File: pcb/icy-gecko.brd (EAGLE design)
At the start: 50.8 x 25.4 mm, 64 parts, among them J1 USB-C, J2 8, J3 8, J4 8, J5 8, J6 4, J7 4, U1 EFM32GG12B8XX_QFN64, U2 ICE40LP384-SG32, U3 MIC23159, U6 SST26VF016B

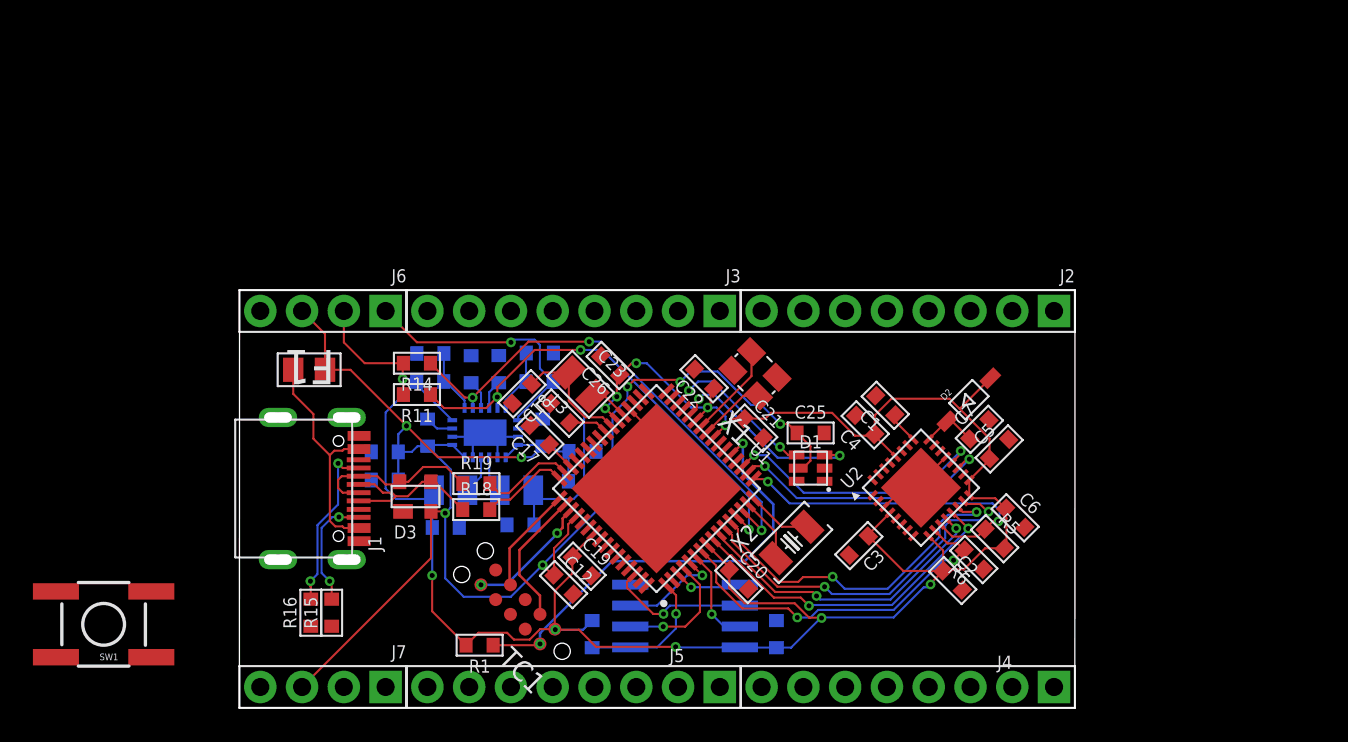
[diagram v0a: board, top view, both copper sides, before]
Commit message: pcd finito
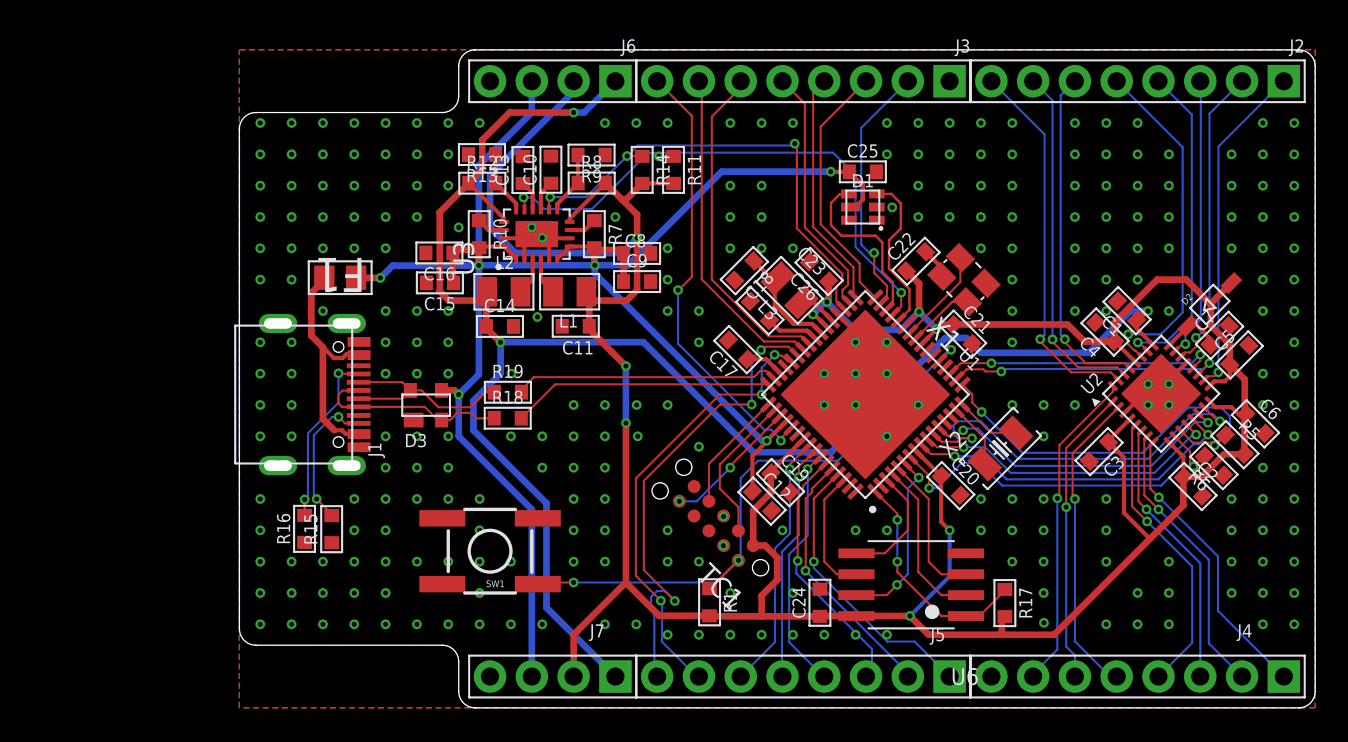
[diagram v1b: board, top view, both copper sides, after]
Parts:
- moved R17 25.2 mm to (46.5, 6.37), flipped to the top, turned to 270 degrees
- moved SW1 23.9 mm to (15.2, 9.53)
- moved R11 20.7 mm to (26.4, 32.7), turned to 270 degrees
- moved J2 19.8 mm to (61.0, 38.1)
- moved J3 19.8 mm to (40.6, 38.1)
- moved J6 19.8 mm to (20.3, 38.1)
- moved C8 19.5 mm to (24.2, 27.6), flipped to the top
- moved C9 19.5 mm to (24.2, 25.9), flipped to the top
- moved R14 18.0 mm to (24.5, 32.7), turned to 270 degrees
- moved C25 16.2 mm to (37.9, 32.6)
- moved D1 16.2 mm to (37.9, 30.4)
- moved C1 15.8 mm to (54.0, 24.1)
- moved R7 15.8 mm to (21.6, 28.8), flipped to the top
- moved D2 15.8 mm to (59.0, 24.5)
- moved C2 15.7 mm to (58.0, 13.5)
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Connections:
- net 1V2_PG: now also U1.29; no longer U1.13
- net 3V3_PG: now also U1.35; no longer U1.14
- net IOL_2A: now also J4.5
- net IOL_2B: now also J4.6
- net IOL_4A: now also J4.4
- net IOL_4B_GBIN7: now also J4.3
- net IOL_5A_GBIN6: now also J4.1
- net IOL_5B: now also J4.2
- net IOR_34: now also J2.1
- net IOR_38: now also J2.2
- net IOR_39: now also J2.3
- net IOT_45: now also J2.4
- net IOT_47: now also J2.5
- net IOT_49_GBIN0: now also J2.6
- net IOT_50_GBIN1: now also J2.7
- net IOT_52: now also J4.7
- net IOT_53: now also J2.8
- net PD3: now also J3.2
- net PD4: now also J3.3
- net PD5: now also J3.4
- net PD6: now also J3.5
- net PE10: now also J5.4
- net PE11: now also J5.3
- net PE12: now also J5.2
- net PE13: now also J5.1
- net PE4: now also J3.6
- net PE5: now also J3.7
- net PE6: now also J5.8
- net PE7: now also J5.7
- net PE8: now also J5.6
- net PE9: now also J5.5
- net PF12: now also J3.8
- net USBDP: now also D3.2; no longer D3.3
- net VUSB: now also D3.3; no longer D3.2
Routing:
- net 1.2V: track 31.1 -> 103.5 mm, vias 1 -> 3
- net 3.3V: track 147.0 -> 203.1 mm, vias 11 -> 9
- net PE6: track 0.00 -> 29.5 mm, vias 0 -> 3
- net PE7: track 0.00 -> 27.4 mm, vias 0 -> 3
- net PF12: track 0.00 -> 27.0 mm, vias 0 -> 2
- net IOT_53: track 0.00 -> 23.0 mm, vias 0 -> 1
- net IOT_50_GBIN1: track 0.00 -> 21.5 mm, vias 0 -> 1
- net IOT_47: track 0.00 -> 21.3 mm, vias 0 -> 1
- net IOT_49_GBIN0: track 0.00 -> 21.0 mm, vias 0 -> 1
- net IOR_34: track 0.00 -> 20.5 mm, vias 0 -> 1
- net PE4: track 0.00 -> 20.3 mm
- net PE5: track 0.00 -> 20.1 mm
- net IOT_45: track 0.00 -> 19.9 mm, vias 0 -> 1
- net IOT_52: track 0.00 -> 19.7 mm, vias 0 -> 1
- net IOL_2A: track 0.00 -> 18.9 mm, vias 0 -> 1
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- added copper zone on layer 1, net GND
- added copper zone on layer 16, net GND
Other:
- board size 50.8 x 25.4 mm -> 65.4 x 40 mm
